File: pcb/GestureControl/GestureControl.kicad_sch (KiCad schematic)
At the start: 71 parts, among them J1 Conn_01x04_I2I-LCD, J2 BATT, J3 Conn_01x08, J4 Conn_01x06, J5 Conn_01x10, J6 Conn_01x08, SW1 SW1, SW2 SW2, U1 AP5100_3.3, U2 AP5100_3.3

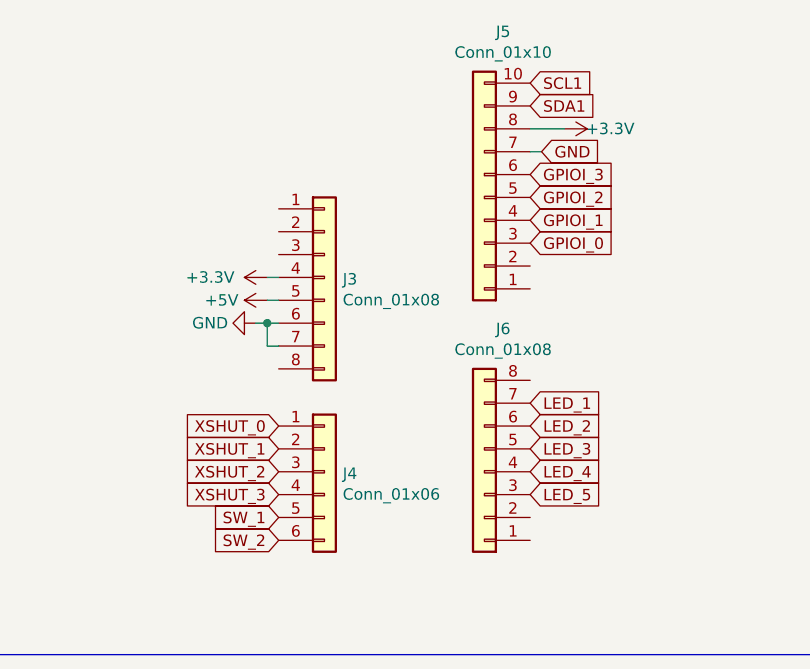
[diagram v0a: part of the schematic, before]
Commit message: add breakoutboard
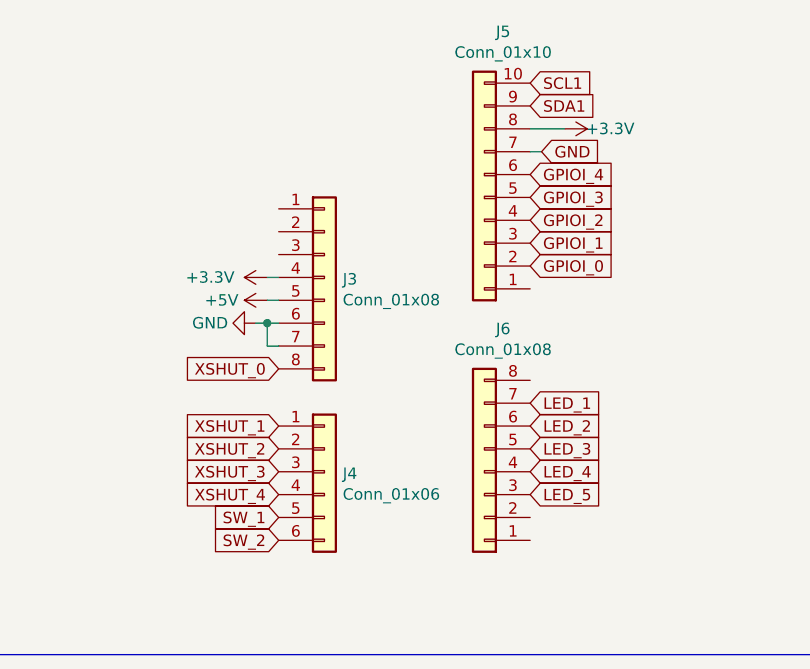
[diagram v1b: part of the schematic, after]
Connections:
- net GPIOI_0: now also J5.2 (Pin_2); no longer J5.3 (Pin_3)
- net GPIOI_1: now also J5.3 (Pin_3); no longer J5.4 (Pin_4)
- net GPIOI_2: now also J5.4 (Pin_4); no longer J5.5 (Pin_5)
- net GPIOI_3: now also J5.5 (Pin_5); no longer J5.6 (Pin_6)
- net XSHUT_0: now also J3.8 (Pin_8); no longer J4.1 (Pin_1)
- net XSHUT_1: now also J4.1 (Pin_1); no longer J4.2 (Pin_2)
- net XSHUT_2: now also J4.2 (Pin_2); no longer J4.3 (Pin_3)
- net XSHUT_3: now also J4.3 (Pin_3); no longer J4.4 (Pin_4)
- new net GPIOI_4: J5.6 (Pin_6)
- new net XSHUT_4: J4.4 (Pin_4)
